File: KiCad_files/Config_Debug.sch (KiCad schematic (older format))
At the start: 50 parts, among them J3 Conn_01x06, J4 USB_C_Receptacle, SW1 SW_Push, U1 XC7A35T_CSG325, U10 W25Q128JV, U6 FT2232HL, U7 93LCxxC, U8 SiT8209, U9 SiT9102, Y1 12MHz

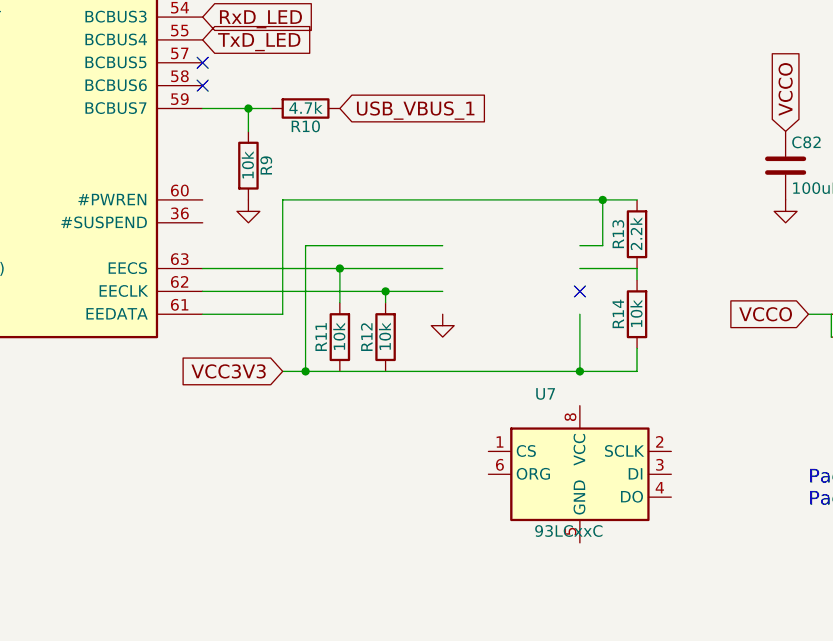
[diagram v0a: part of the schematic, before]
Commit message: More fixes
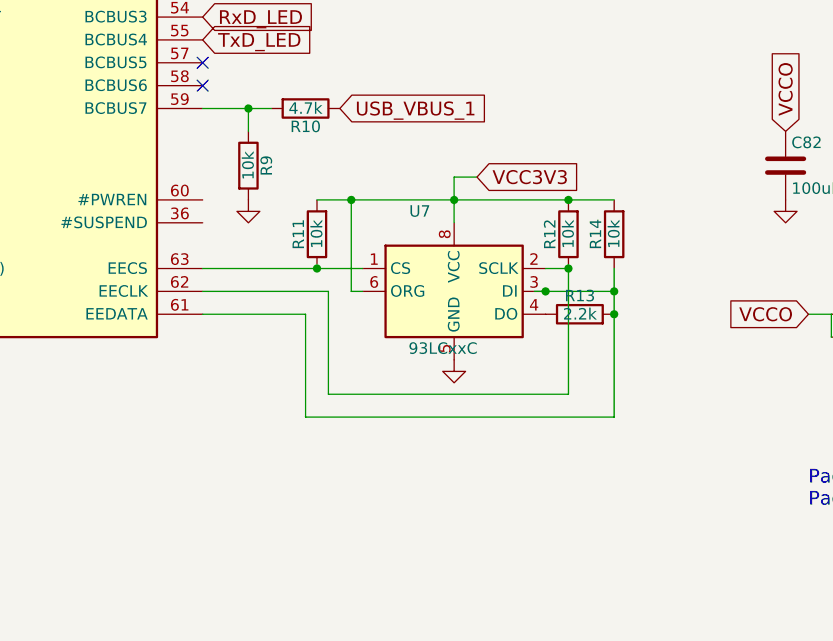
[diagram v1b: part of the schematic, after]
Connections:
- wire segments 229 -> 232
- no-connect marks 24 -> 23
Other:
- moved on the sheet: R11, R12, R13, R14, U7
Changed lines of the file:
@@
 L Memory_EEPROM:93LCxxC U7
 U 1 1 5C194DEC
-P 6500 6200
+P 5950 5400
 AR Path="/5C194DEC" Ref="U7"  Part="1"
 AR Path="/5C0630AC/5C194DEC" Ref="U7"  Part="1"
-F 0 "U7" H 6350 6550 50  0000 C CNN
-F 1 "93LCxxC" H 6300 5950 50  0000 L CNN
-F 2 "" H 6400 6200 50  0001 C CNN
-F 3 "" H 6500 6300 50  0001 C CNN
-	1    6500 6200
+F 0 "U7" H 5800 5750 50  0000 C CNN
+F 1 "93LCxxC" H 5750 5150 50  0000 L CNN
+F 2 "" H 5850 5400 50  0001 C CNN
+F 3 "" H 5950 5500 50  0001 C CNN
+	1    5950 5400
 	1    0    0    -1
 $EndComp
@@
 L Device:R R13
 U 1 1 5C194DF3
-P 6750 5150
-F 0 "R13" V 6830 5150 50  0000 C CNN
-F 1 "2.2k" V 6750 5150 50  0000 C CNN
-F 2 "" V 6680 5150 50  0001 C CNN
-F 3 "" H 6750 5150 50  0001 C CNN
-	1    6750 5150
-	-1   0    0    1
-$EndComp
-Text GLabel 5200 5750 0    60   Input ~ 0
+P 6500 5500
+F 0 "R13" V 6580 5500 50  0000 C CNN
+F 1 "2.2k" V 6500 5500 50  0000 C CNN
+F 2 "" V 6430 5500 50  0001 C CNN
+F 3 "" H 6500 5500 50  0001 C CNN
+	1    6500 5500
+	0    -1   -1   0
+$EndComp
+Text GLabel 6050 4900 2    60   Input ~ 0
 VCC3V3
 $Comp
 L Device:R R12
 U 1 1 5C194DFB
-P 5650 5600
-F 0 "R12" V 5730 5600 50  0000 C CNN
-F 1 "10k" V 5650 5600 50  0000 C CNN
-F 2 "" V 5580 5600 50  0001 C CNN
-F 3 "" H 5650 5600 50  0001 C CNN
-	1    5650 5600
+P 6450 5150
+F 0 "R12" V 6530 5150 50  0000 C CNN
+F 1 "10k" V 6450 5150 50  0000 C CNN
+F 2 "" V 6380 5150 50  0001 C CNN
+F 3 "" H 6450 5150 50  0001 C CNN
+	1    6450 5150
 	-1   0    0    1
 $EndComp
@@
 L Device:R R11
 U 1 1 5C194E02
-P 5450 5600
-F 0 "R11" V 5530 5600 50  0000 C CNN
-F 1 "10k" V 5450 5600 50  0000 C CNN
-F 2 "" V 5380 5600 50  0001 C CNN
-F 3 "" H 5450 5600 50  0001 C CNN
-	1    5450 5600
+P 5350 5150
+F 0 "R11" V 5430 5150 50  0000 C CNN
+F 1 "10k" V 5350 5150 50  0000 C CNN
+F 2 "" V 5280 5150 50  0001 C CNN
+F 3 "" H 5350 5150 50  0001 C CNN
+	1    5350 5150
 	-1   0    0    1
 $EndComp
@@
 L Device:R R14
 U 1 1 5C194E09
-P 6750 5500
-F 0 "R14" V 6830 5500 50  0000 C CNN
-F 1 "10k" V 6750 5500 50  0000 C CNN
-F 2 "" V 6680 5500 50  0001 C CNN
-F 3 "" H 6750 5500 50  0001 C CNN
-	1    6750 5500
+P 6650 5150
+F 0 "R14" V 6730 5150 50  0000 C CNN
+F 1 "10k" V 6650 5150 50  0000 C CNN
+F 2 "" V 6580 5150 50  0001 C CNN
+F 3 "" H 6650 5150 50  0001 C CNN
+	1    6650 5150
 	-1   0    0    1
 $EndComp
@@
 	6450 2850 6450 2800
 Connection ~ 6200 2850
-Wire Wire Line
-	4850 5300 5450 5300
-Wire Wire Line
-	4850 5400 5650 5400
-Wire Wire Line
-	6500 5200 6600 5200
-Wire Wire Line
-	6600 5200 6600 5000
-Wire Wire Line
-	5200 5000 6600 5000
-Wire Wire Line
-	5200 5000 5200 5500
-Wire Wire Line
-	5200 5500 4850 5500
-Connection ~ 6600 5000
-Wire Wire Line
-	6500 5300 6750 5300
-Wire Wire Line
-	5900 5200 5300 5200
-Wire Wire Line
-	5300 5200 5300 5750
-Wire Wire Line
-	5200 5750 5300 5750
-Wire Wire Line
-	5650 5450 5650 5400
-Connection ~ 5650 5400
-Wire Wire Line
-	5450 5300 5450 5450
-Connection ~ 5450 5300
-Connection ~ 5300 5750
-Wire Wire Line
-	6500 5750 6500 5500
-Connection ~ 6500 5750
-NoConn ~ 6500 5400
-Wire Wire Line
-	6750 5300 6750 5350
-Wire Wire Line
-	6750 5750 6750 5650
 $Comp
 L power:GND #PWR079
 U 1 1 5C194EA2
-P 5900 5500
-F 0 "#PWR079" H 5900 5250 50  0001 C CNN
-F 1 "GND" H 5900 5350 50  0001 C CNN
-F 2 "" H 5900 5500 50  0001 C CNN
-F 3 "" H 5900 5500 50  0001 C CNN
-	1    5900 5500
+P 5950 5700
+F 0 "#PWR079" H 5950 5450 50  0001 C CNN
+F 1 "GND" H 5950 5550 50  0001 C CNN
+F 2 "" H 5950 5700 50  0001 C CNN
+F 3 "" H 5950 5700 50  0001 C CNN
+	1    5950 5700
 	1    0    0    -1
 $EndComp
@@
 Wire Wire Line
 	6200 2850 6450 2850
-Wire Wire Line
-	6600 5000 6750 5000
-Wire Wire Line
-	5650 5400 5900 5400
-Wire Wire Line
-	5450 5300 5900 5300
-Wire Wire Line
-	5300 5750 6500 5750
-Wire Wire Line
-	6500 5750 6750 5750
 $Comp
 L Connector:USB_C_Receptacle_USB2.0 J4
@@
 NoConn ~ 4850 4400
 NoConn ~ 4850 4500
+Wire Wire Line
+	5950 5000 5500 5000
+Wire Wire Line
+	5500 5400 5550 5400
+Connection ~ 5950 5000
+Wire Wire Line
+	5550 5300 5350 5300
+Wire Wire Line
+	4850 5400 5400 5400
+Wire Wire Line
+	5400 5400 5400 5850
+Wire Wire Line
+	5400 5850 6450 5850
+Wire Wire Line
+	6450 5850 6450 5300
+Wire Wire Line
+	6450 5300 6350 5300
+Wire Wire Line
+	6300 5400 6350 5400
+Wire Wire Line
+	6650 5400 6650 5500
+Wire Wire Line
+	6650 5950 5300 5950
+Wire Wire Line
+	5300 5950 5300 5500
+Wire Wire Line
+	5300 5500 4850 5500
+Connection ~ 5350 5300
+Wire Wire Line
+	5350 5300 4850 5300
+Wire Wire Line
+	5500 5000 5500 5400
+Wire Wire Line
+	5950 5000 5950 5100
+Wire Wire Line
+	5500 5000 5350 5000
+Connection ~ 5500 5000
+Connection ~ 6450 5300
+Wire Wire Line
+	6650 5300 6650 5400
+Connection ~ 6650 5400
+Connection ~ 6450 5000
+Wire Wire Line
+	6050 4900 5950 4900
+Wire Wire Line
+	5950 4900 5950 5000
+Connection ~ 6350 5400
+Wire Wire Line
+	6350 5400 6650 5400
+Connection ~ 6650 5500
+Wire Wire Line
+	6650 5500 6650 5950
+Wire Wire Line
+	6450 5000 6650 5000
+Wire Wire Line
+	5950 5000 6450 5000
 $EndSCHEMATC
